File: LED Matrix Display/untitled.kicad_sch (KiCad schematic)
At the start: 1 part

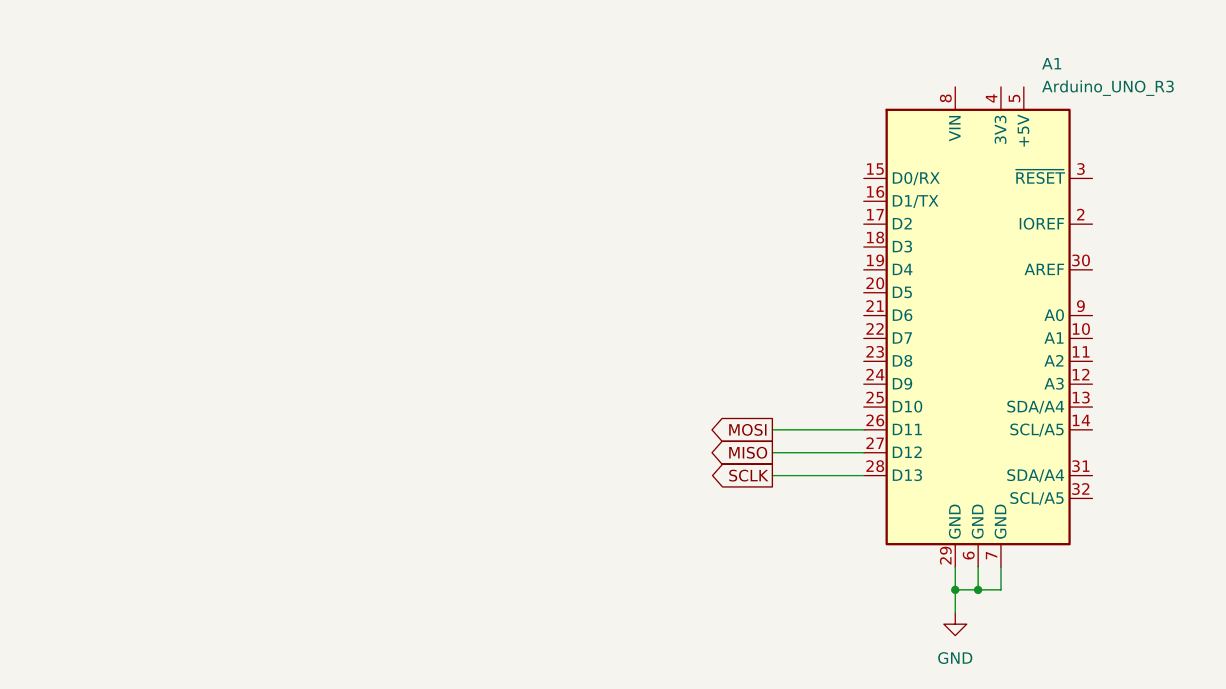
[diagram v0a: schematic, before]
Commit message: SCH and PCB updates
Added updates to SCH and made progress on layout.
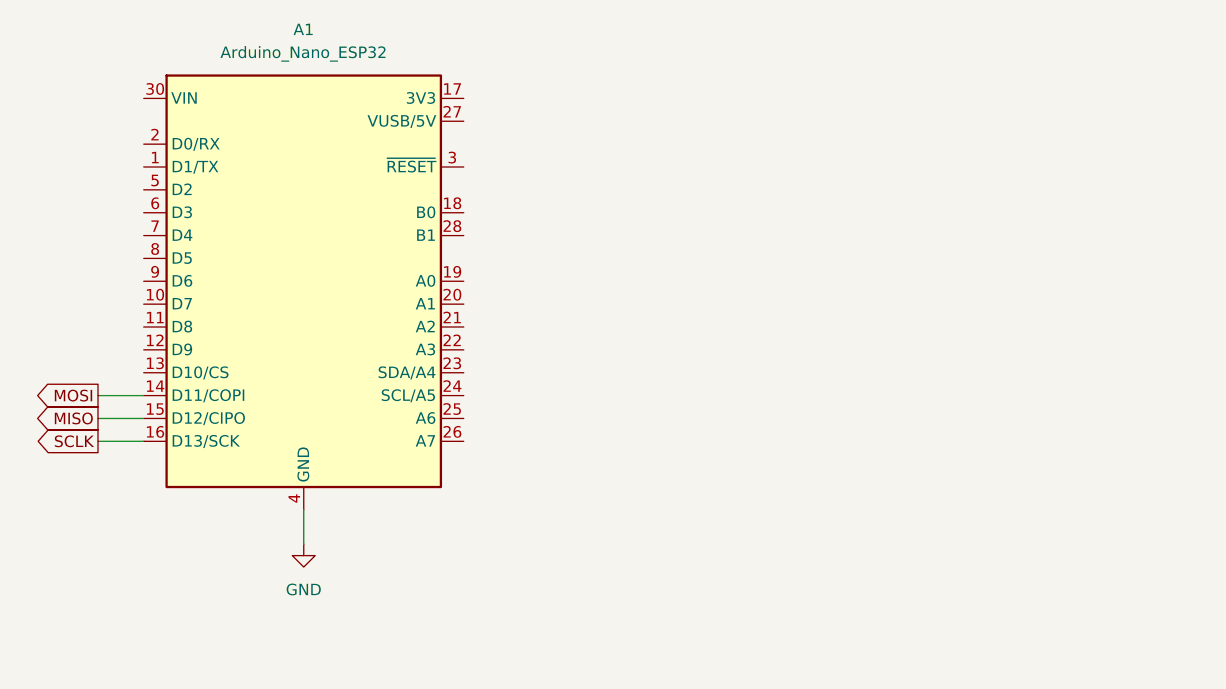
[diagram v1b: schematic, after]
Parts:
- removed A1: Arduino_UNO_R3, Module:Arduino_UNO_R3, symbol MCU_Module:Arduino_UNO_R3
- added A1: Arduino_Nano_ESP32, Module:Arduino_Nano, symbol MCU_Module:Arduino_Nano_ESP32
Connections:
- net GND: now also A1.29 (GND), A1.4 (GND)
- net MISO: now also A1.15 (D12/CIPO)
- net MOSI: now also A1.14 (D11/COPI)
- net SCLK: now also A1.16 (D13/SCK)
